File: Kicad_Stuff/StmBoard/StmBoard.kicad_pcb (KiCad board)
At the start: 2 copper layers, 46 parts, among them J1 USB_B_Mini, SW1 SW_DIP_x01, SW2 SW_DIP_x01, SW3 SW_DIP_x01, SW4 SW_DIP_x01, SW5 SW_DIP_x01, SW6 SW_DIP_x01, SW7 SW_DIP_x01, SW8 SW_DIP_x01, SW9 SW_DIP_x01, U1 STM32G031K8Tx, U13 MCP2221AxST, U2 LIS3DH, U8 MIC5504-3.3YM5, U9 L78L05_SO8, Y1 32Khz LSE

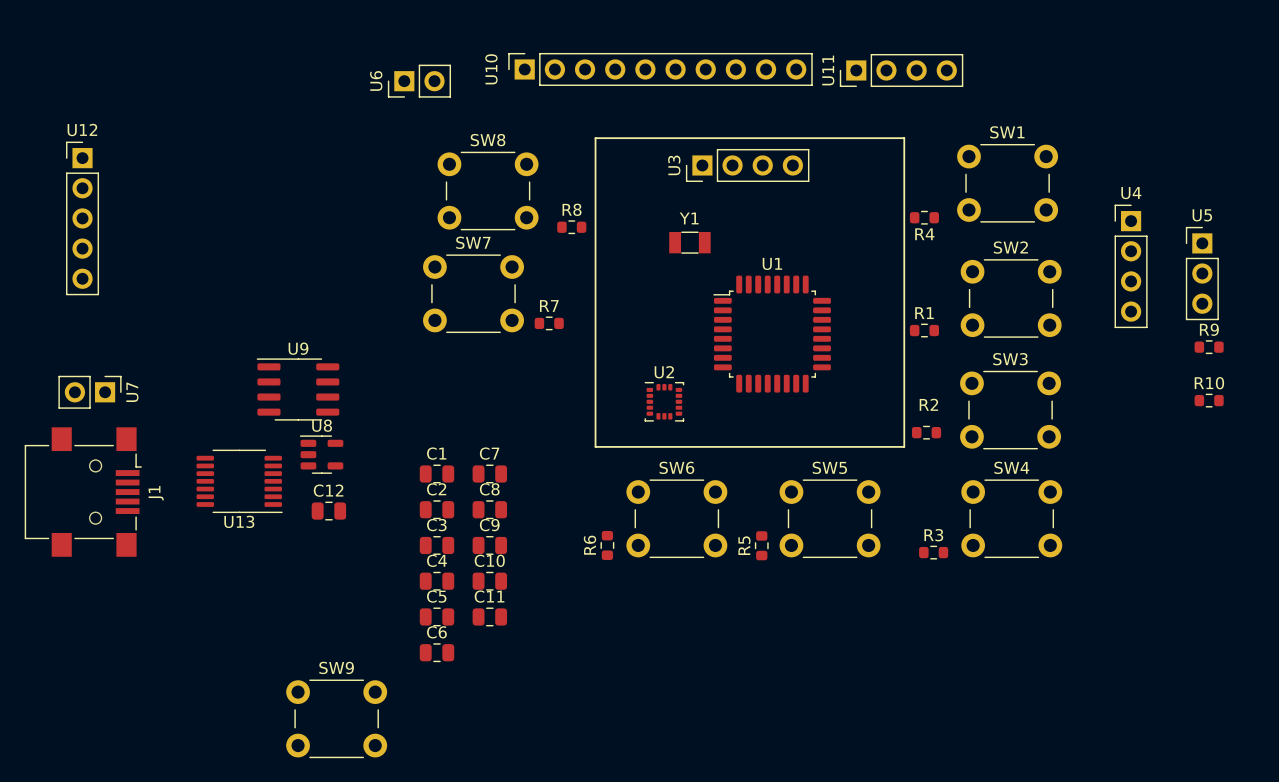
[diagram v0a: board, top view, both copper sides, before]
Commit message: quick commit
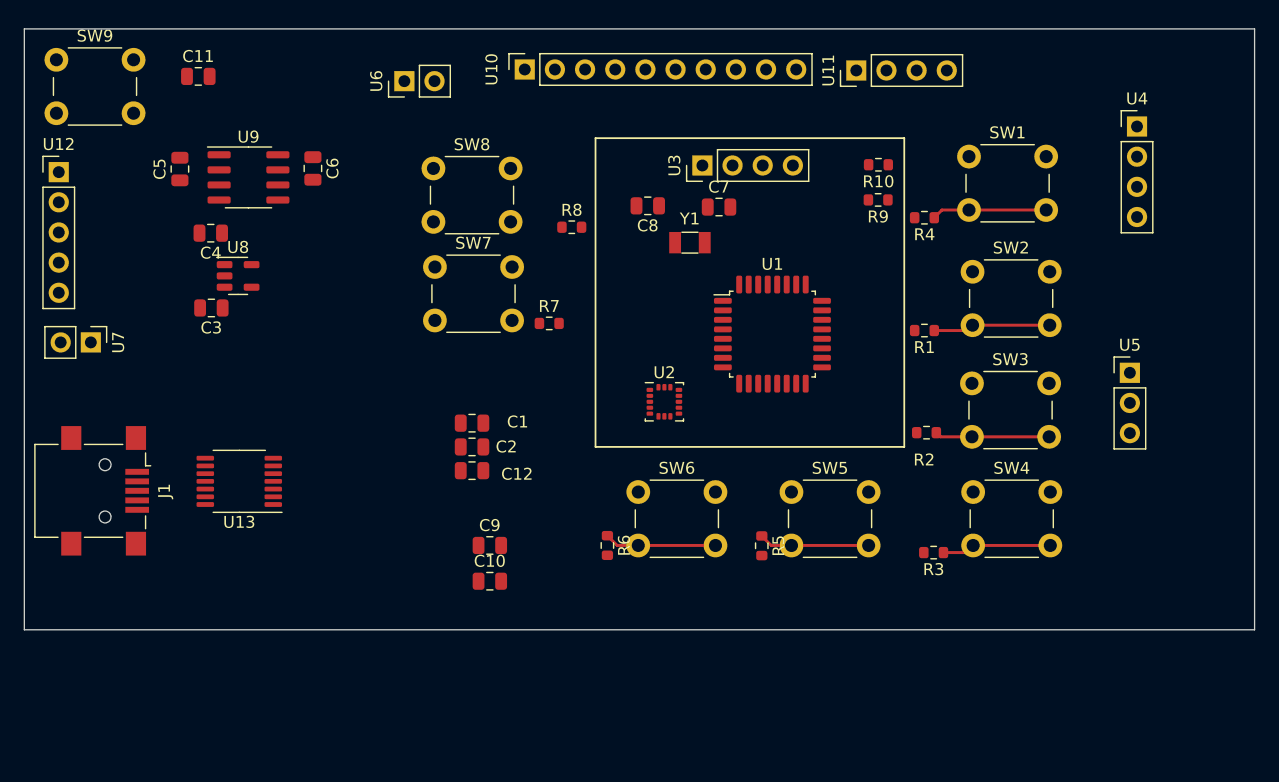
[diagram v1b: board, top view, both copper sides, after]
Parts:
- moved SW9 57.0 mm to (77.4, 78.7)
- moved C11 51.7 mm to (89.3, 80.1)
- moved C5 43.5 mm to (87.8, 87.9), turned to 90 degrees
- moved C6 42.1 mm to (99.0, 87.8), turned to -90 degrees
- moved C4 35.0 mm to (90.4, 93.3), turned to 180 degrees
- moved R10 34.2 mm to (146.6, 87.5), turned to 180 degrees
- moved R9 30.5 mm to (146.6, 90.5), turned to 180 degrees
- moved C7 29.6 mm to (133.2, 91.1)
- moved C8 28.8 mm to (127.2, 91.0), turned to 180 degrees
- moved C3 27.6 mm to (90.5, 99.6), turned to 180 degrees
- moved U9 18.3 mm to (93.6, 88.6)
- moved U8 16.6 mm to (92.7, 96.9)
- moved C12 12.5 mm to (112.4, 113.3)
- moved U5 12.5 mm to (167.8, 105.1)
- moved U4 7.98 mm to (168.4, 84.3)
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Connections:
- U10 pad 10: (no net) -> Net-(U1-PB0)
- U12 pad 1: (no net) -> GND
- U12 pad 2: (no net) -> VCC
- U12 pad 3: (no net) -> /reset
- U12 pad 4: (no net) -> SWCLK
- U12 pad 5: (no net) -> SWDIO
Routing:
- net /A1: track 0.00 -> 10.1 mm
- net /A0: track 0.00 -> 9.69 mm
- net /A2: track 0.00 -> 9.64 mm
- net /A4: track 0.00 -> 9.58 mm
- net /A5: track 0.00 -> 9.44 mm
- net /A3: track 0.00 -> 9.25 mm
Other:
- board outline added: 103.6 x 50.6 mm
- copper layers 2 -> 4
